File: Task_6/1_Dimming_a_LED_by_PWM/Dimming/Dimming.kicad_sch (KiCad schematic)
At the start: 6 parts, among them Q1 BC817

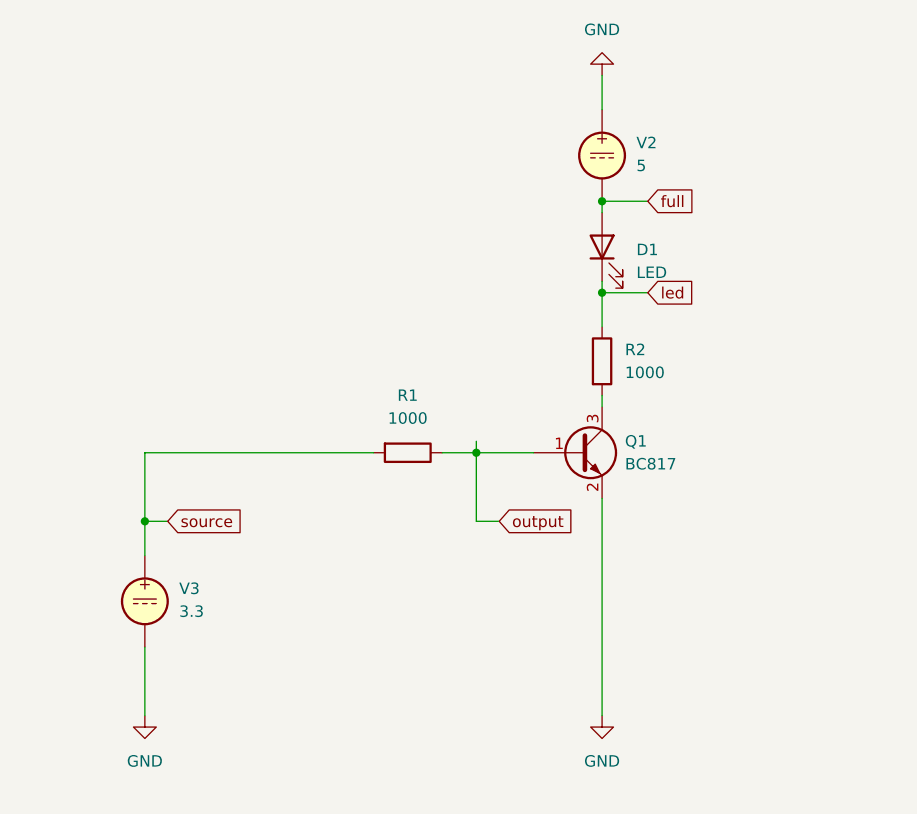
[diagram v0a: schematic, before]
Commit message: Completed 6) Simulation and Measurement
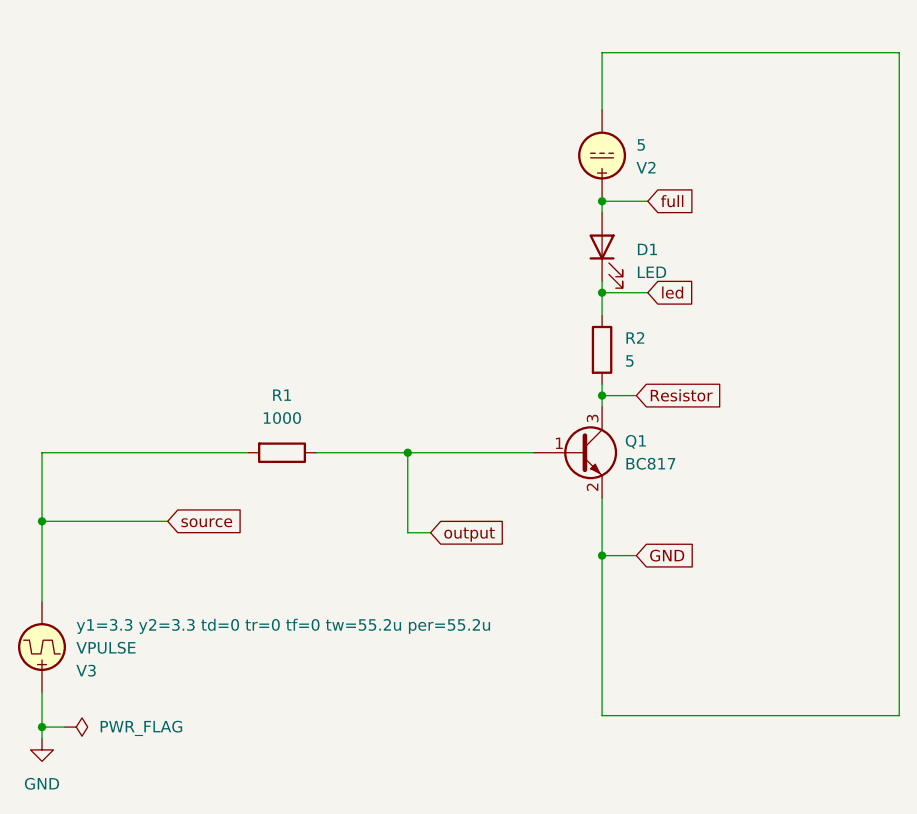
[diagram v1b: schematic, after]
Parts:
- removed V3: 3.3, symbol Simulation_SPICE:VDC
- added V3: VPULSE, symbol Simulation_SPICE:VPULSE
- R2: value 1000 -> 5
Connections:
- net GND: now also V2.2, V3.1; no longer V2.1
- net full: now also V2.1; no longer V2.2
- net source: now also V3.2
- net Resistor: now reaches Q1.3 (C), R2.2
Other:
- moved on the sheet: R1, R2
